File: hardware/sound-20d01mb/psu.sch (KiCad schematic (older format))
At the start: 6 parts

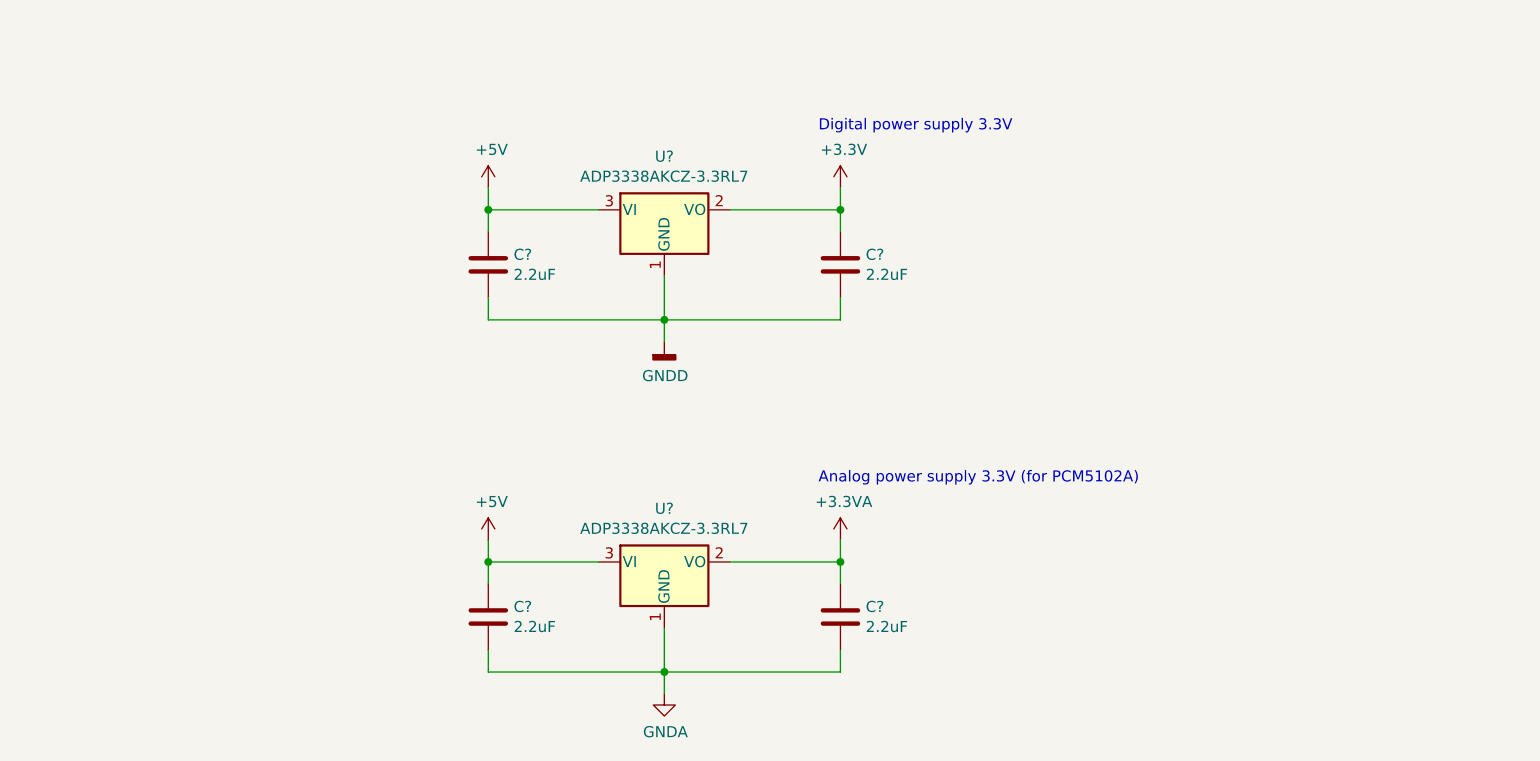
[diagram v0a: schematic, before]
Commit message: Updated PSU
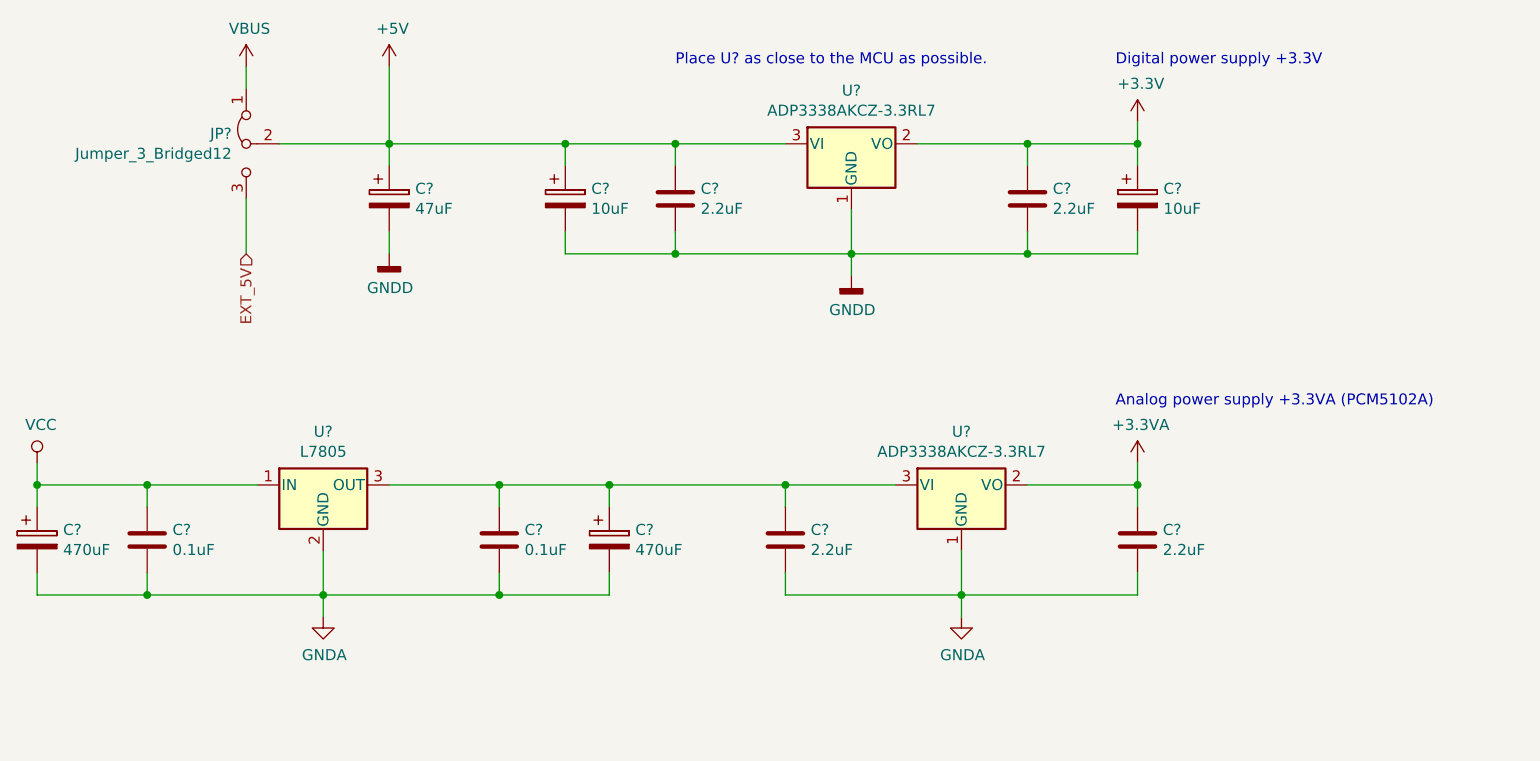
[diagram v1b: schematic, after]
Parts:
- added C?: 47uF, symbol Device:CP
- added C? (x2): 10uF, symbol Device:CP
- added C? (x2): 470uF, symbol Device:CP
- added C? (x2): 0.1uF, Capacitor_SMD:C_1206_3216Metric_Pad1.42x1.75mm_HandSolder, symbol Device:C
- added JP?: Jumper_3_Bridged12, Connector_PinHeader_2.54mm:PinHeader_1x03_P2.54mm_Vertical, symbol Jumper:Jumper_3_Bridged12
- added U?: L7805, symbol Regulator_Linear:L7805
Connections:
- net +3V3: now also C?.1
- net +5V: now also C?.1, C?.1, JP?.2 (C); no longer C?.1, U?.3 (VI)
- net GNDA: now also C?.2, C?.2, C?.2, C?.2, U?.2 (GND)
- net GNDD: now also C?.2, C?.2, C?.2
- new net: C?.1, C?.1, C?.1, U?.3 (OUT), U?.3 (VI)
- new net EXT_5V: JP?.3 (B)
- new net VBUS: JP?.1 (A)
- new net VCC: C?.1, C?.1, U?.1 (IN)
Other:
- note added: "Analog power supply +3.3VA (PCM5102A)"
- note added: "Digital power supply +3.3V"
- note added: "Place U? as close to the MCU as possible."
- note removed: "Analog power supply 3.3V (for PCM5102A)"
- note removed: "Digital power supply 3.3V"
- moved on the sheet: C?, U?
